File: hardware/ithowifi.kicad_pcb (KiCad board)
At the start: 2 copper layers, 42.3 x 45.1 mm, 32 parts, among them J1 CONN_01X07, J2 conn, J3 Conn_Coaxial, J4 Conn_01x04, Q1 BSS138, Q2 BSS138, U1 ESP32-WROOM, U2 CC1101-868MHz-Module, U3 AMS1117-3.3

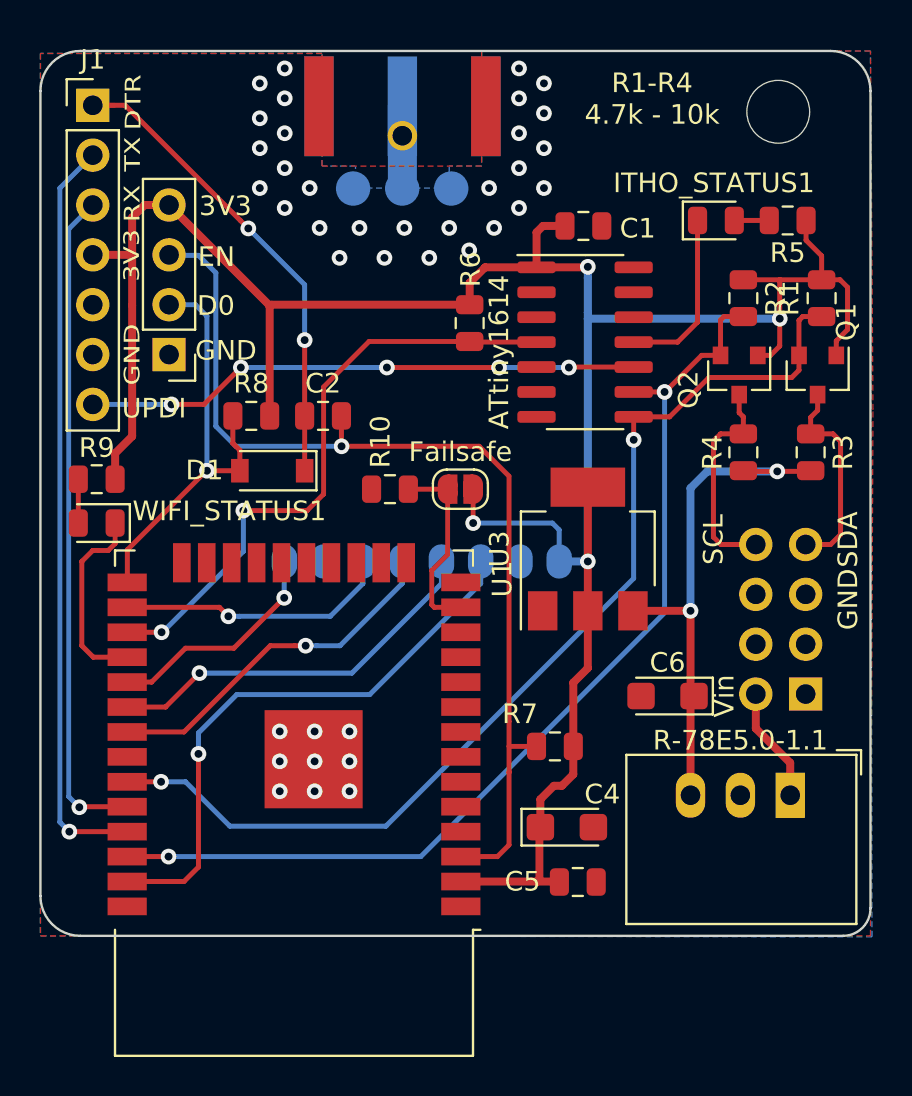
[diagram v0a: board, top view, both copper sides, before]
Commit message: Update PCB files Change C to HTML Celcius Small CC1101 lib cleanup Update attiny firmware files
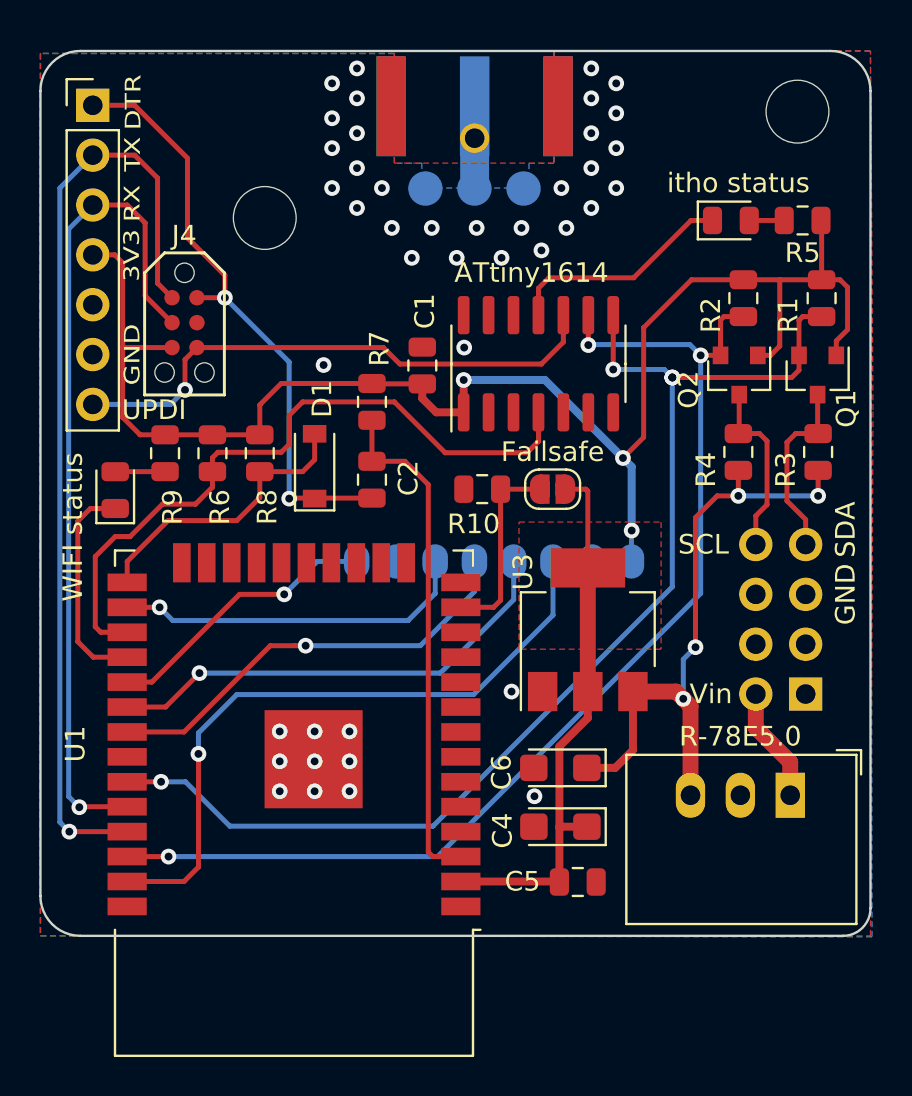
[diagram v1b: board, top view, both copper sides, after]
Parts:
- removed ITHO_STATUS1, WIFI_STATUS1: LED, LED_SMD:LED_0805_2012Metric
- added H2: MountingHole, MountingHole:MountingHole_2.5mm, F.Cu at (94.5, 113.5)
- added LED1: WIFI status, LED_SMD:LED_0805_2012Metric, F.Cu at (86.9, 127.4)
- added LED2: itho status, LED_SMD:LED_0805_2012Metric, F.Cu at (118.2, 113.7)
- J4: value Conn_01x04 -> TC2030-MCP-NL; footprint Connector_PinHeader_2.54mm:PinHeader_1x04_P2.54mm_Vertical -> nrg_watch:TC2020-MCP-NL
- moved R7 19.9 mm to (99.9, 122.9), turned to 90 degrees
- moved R6 14.7 mm to (91.8, 125.5)
- moved C1 10.9 mm to (102.5, 121.1), turned to 90 degrees
- moved C6 6.57 mm to (109.5, 141.6)
- moved JP1 4.70 mm to (109.2, 127.4)
- moved R10 4.70 mm to (105.6, 127.4)
- moved U3 4.11 mm to (110.9, 134.5)
- moved C2 4.10 mm to (99.9, 126.9), turned to 270 degrees
- moved R9 3.72 mm to (89.4, 125.5), turned to 270 degrees
- moved REF** 3.69 mm to (105.2, 109.5)
- moved J3 3.68 mm to (105.2, 107.8)
- moved U2 3.68 mm to (106.2, 121.5)
- moved ATtiny1614 2.62 mm to (108.4, 121.0), turned to 90 degrees
- moved D1 2.17 mm to (97.0, 126.2), turned to 90 degrees
- moved R8 1.95 mm to (94.2, 125.5), turned to 90 degrees
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- renumbered R-78E5.0-1.1 to R-78E5.0
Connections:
- C2 pad 2: Net-(C2-Pad2) -> DTR
- D1 pad 1: Net-(C2-Pad2) -> DTR
- J1 pad 1: Net-(C2-Pad2) -> DTR
- J4 pad 1: GND -> D1/TX0
- J4 pad 2: D0 -> DTR
- J4 pad 3: EN -> D0/RX0
- J4 pad 4: +3V3 -> GND
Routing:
- net DTR: track 0.00 -> 31.1 mm, vias 0 -> 2
- net Net-(C2-Pad2): track 25.2 -> 0.00 mm, vias 2 -> 0
- net EN: track 51.1 -> 25.9 mm, vias 1 -> 0
- net +3V3: track 129.6 -> 108.0 mm, vias 4 -> 3
- net D1/TX0: track 38.3 -> 48.5 mm
- net D0/RX0: track 34.1 -> 42.6 mm
- net Net-(ATtiny1614-Pad8): track 53.4 -> 60.8 mm, vias 2 -> 4
- net D0: track 22.1 -> 14.9 mm, vias 1 -> 0
- net Net-(ATtiny1614-Pad9): track 52.0 -> 58.4 mm, vias 2 -> 3
- net +5V: track 26.8 -> 32.3 mm, vias 2 -> 4
- net D23_MOSI: track 29.4 -> 34.1 mm
- net Net-(ATtiny1614-Pad4): track 31.4 -> 35.7 mm, vias 2 -> 0
- net D18_SCK: track 19.7 -> 23.9 mm
- net D4_IRQ: track 14.0 -> 18.2 mm
- net D19_MISO: track 18.3 -> 22.2 mm
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- added copper zone on F.Cu, net +3V3
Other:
- copper layers 2 -> 4
- board text added: "Itho CVE ESP WiFi Controller v2.4 Arjen Hiemstra - GNU GPL 3.0"
- board text removed: "D0"
- board text removed: "EN"
- board text removed: "Itho CVE ESP WiFi Controller v2.2 Arjen Hiemstra - GNU GPL 3.0"
- board text removed: "R1-R4 4.7k - 10k"
